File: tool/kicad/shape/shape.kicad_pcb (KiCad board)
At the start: 2 copper layers, 19.3 x 20 mm, 29 parts, among them K1 CONN_3, P1 CONN_7, U1 MCP6022

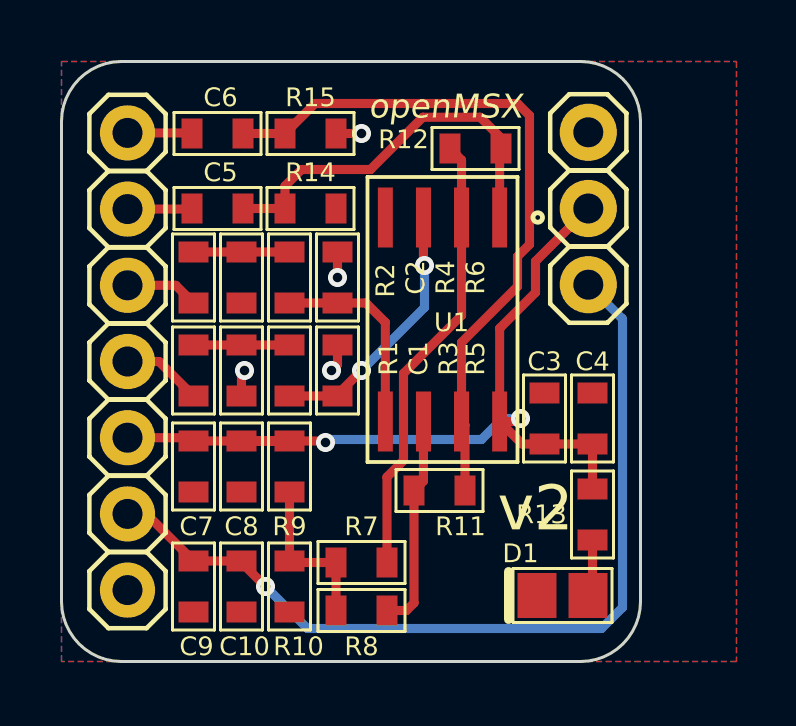
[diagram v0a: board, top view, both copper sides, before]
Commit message: tune shape board
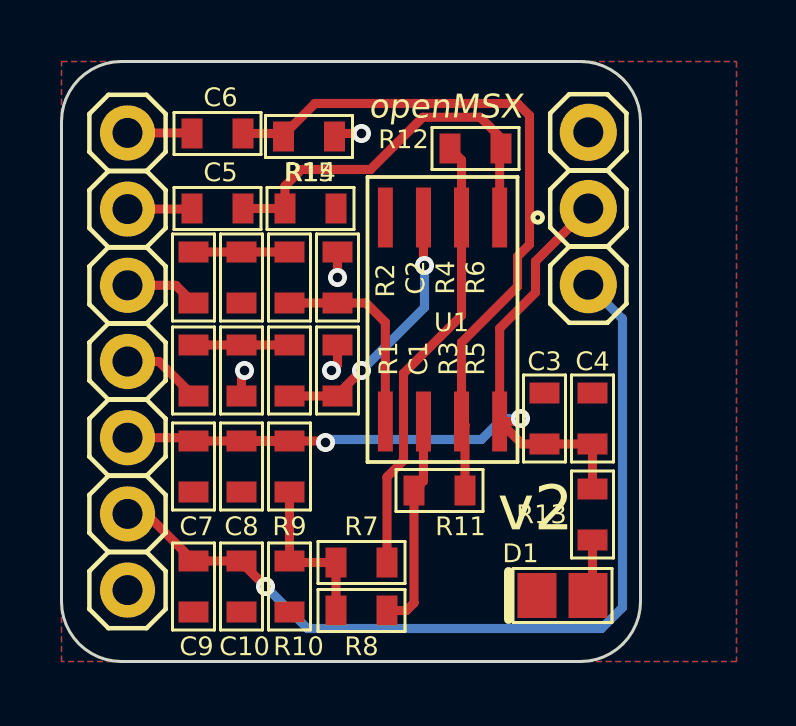
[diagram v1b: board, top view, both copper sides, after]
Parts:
- C5, C6: value 0.1uF -> 0Ohm
- R1, R2: value 2.2k -> 0/2.2k
- R10: value 1.5k -> 1.21k
- R14, R15: value 100 -> NC
- R3, R4, R7, R8: value 22k -> 68k
- R9: value 1k -> 1.5k
- moved R15 0.11 mm to (73.2, 92.5), turned to 0 degrees
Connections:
- R15 pad 1: GND -> /ROO
- R15 pad 2: /ROO -> GND
